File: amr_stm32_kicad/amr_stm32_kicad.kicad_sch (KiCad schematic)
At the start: 98 parts, among them J1 Header 2x20, J10 VCC, J2 Motor_Left, J3 Motor_right, J4 ST_Link, J5 USB_FS_Interface, J6 USB_UART, J7 +12V_BAT, J8 USB_A_Pi, J9 UART, Q1 FDN304P, SW1 SW_Reset, SW2 SW_BOOT, U1 SGM2205_3.3, U3 BMI323, U4 TB6612FNG, U5 STM32F405RGTx, U6 LMV358, U7 CH340E, U9 TPS56528DDA, Y2 8MHz

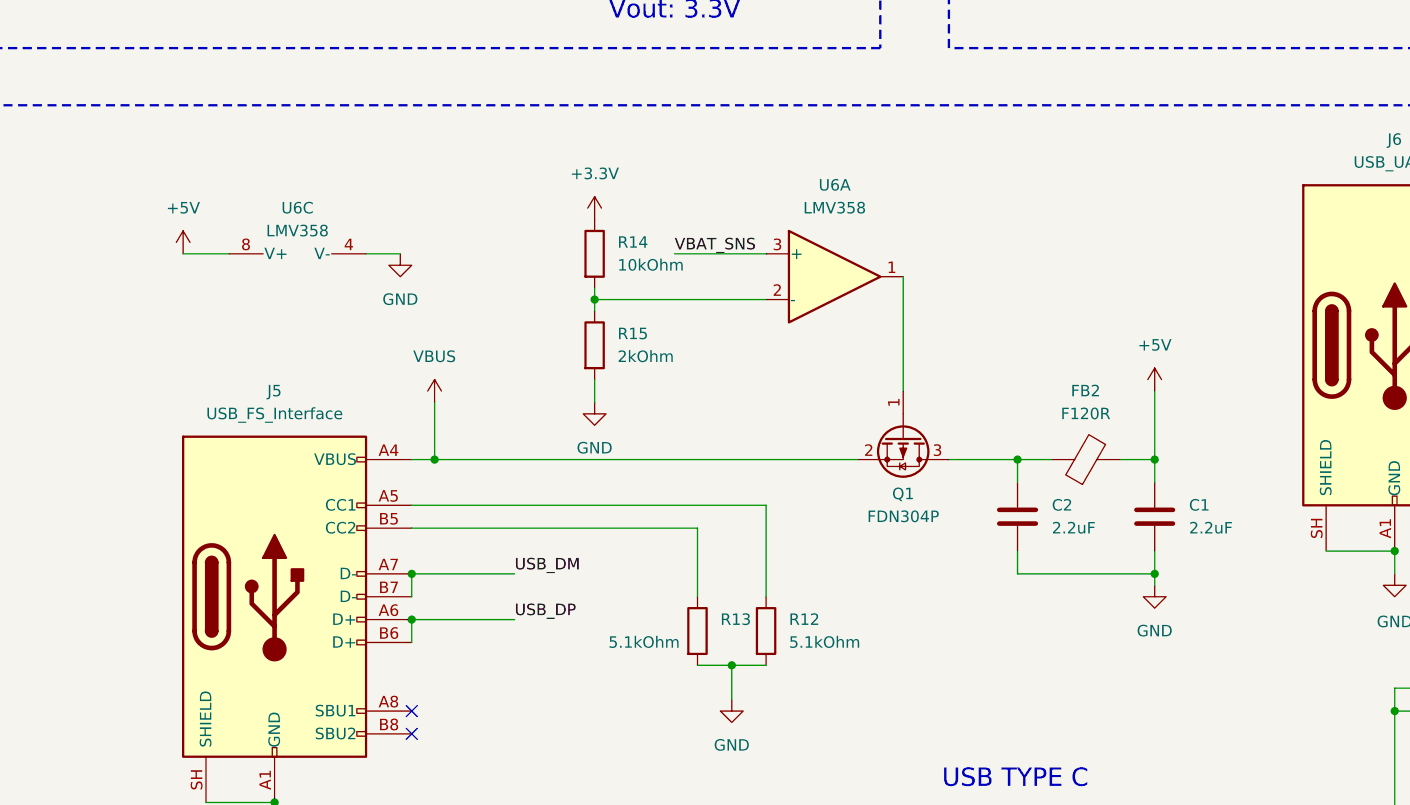
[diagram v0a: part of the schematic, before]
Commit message: update9_10
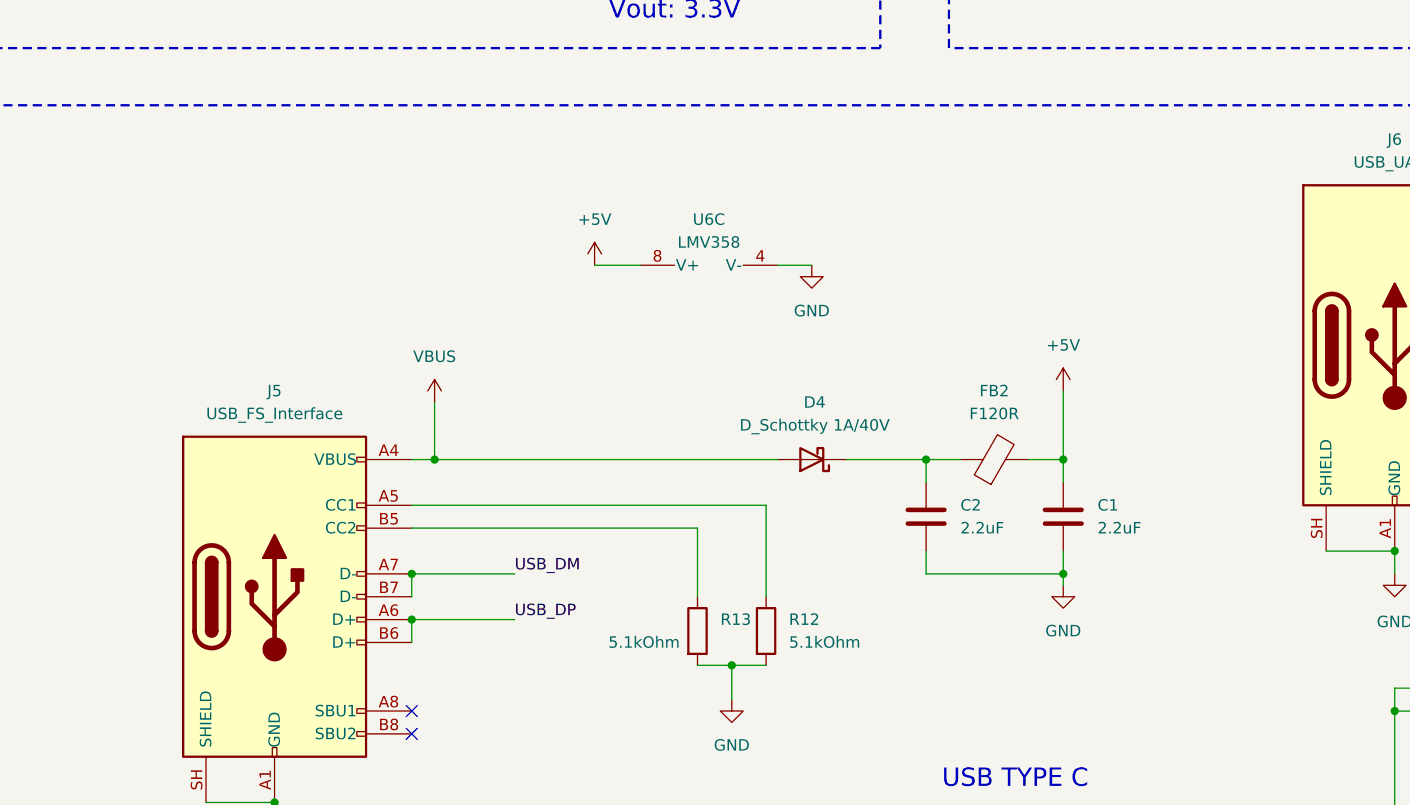
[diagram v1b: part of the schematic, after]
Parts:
- removed Q1: FDN304P, Package_TO_SOT_SMD:SOT-23, symbol Transistor_FET:Q_PMOS_GSD
- removed R14: 10kOhm, Resistor_SMD:R_0603_1608Metric, symbol Device:R
- removed R15: 2kOhm, Resistor_SMD:R_0603_1608Metric, symbol Device:R
- removed unit 1 of U6
- added D4: D_Schottky 1A/40V, Diode_SMD:D_SOD-123, symbol Device:D_Schottky
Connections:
- net VBUS: now also D4.2 (A)
- net at C2.1, FB2.1: now also D4.1 (K)
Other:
- moved on the sheet: C1, C2, FB2, U6C
